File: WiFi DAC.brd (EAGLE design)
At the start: 65 x 30 mm, 27 parts

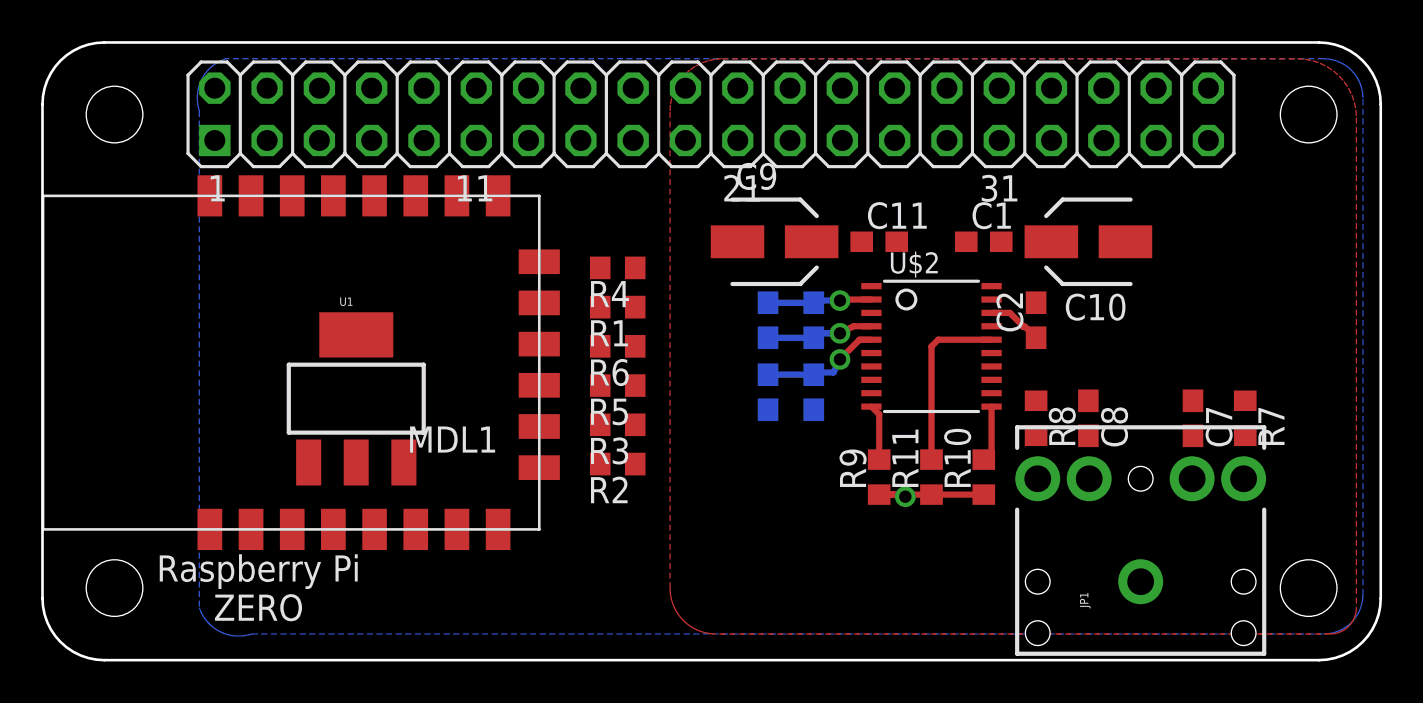
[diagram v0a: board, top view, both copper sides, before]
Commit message: test
jup
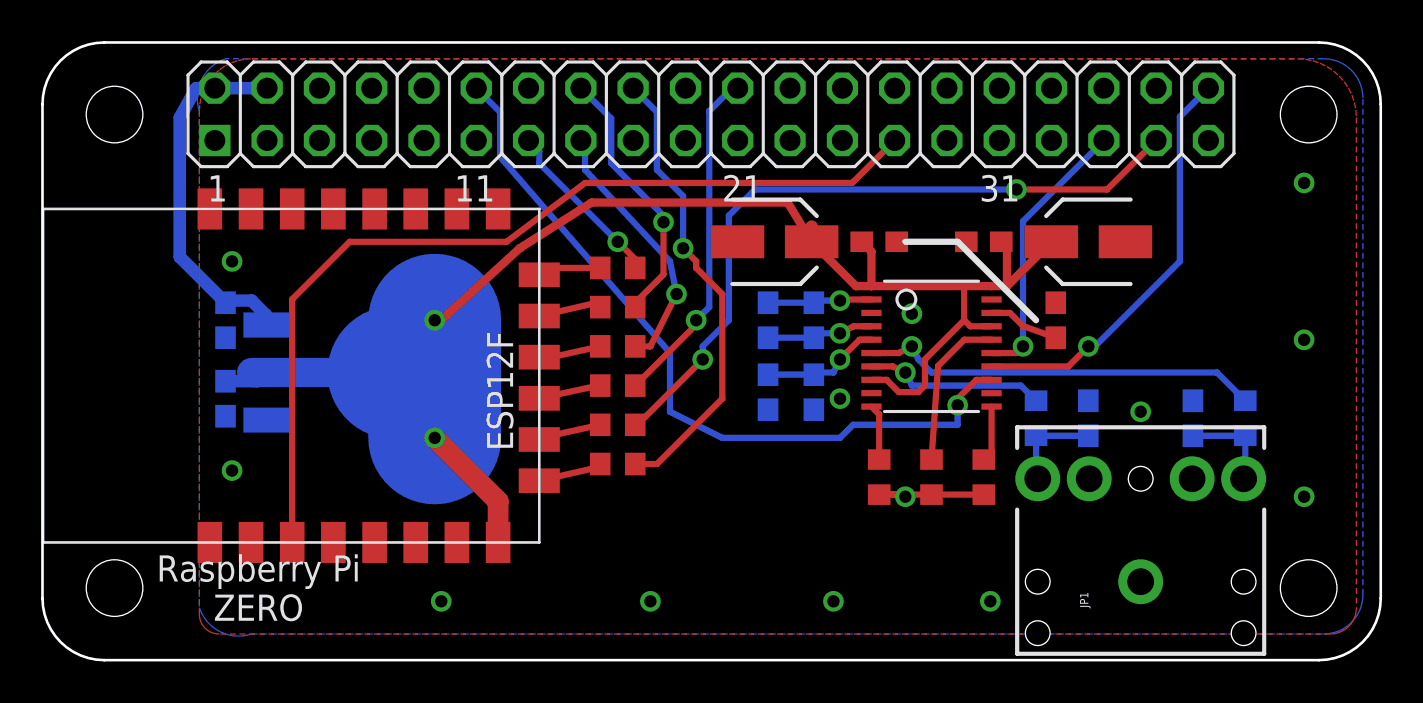
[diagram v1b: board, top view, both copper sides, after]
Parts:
- added C12: 2x 100nF, rcl:C0603
- added C13: 100nF, rcl:C0603
- C11: value 100nF -> 3x 100nF
- C4: value 100nF -> 2x 100nF
- C5: value 2.2uF -> 2x 2.2uF
- R2: value 33 -> 6x 33
- R4: value 33 -> 6x 33R
- R9: value 47k -> 3x 47k
- moved U1 1.80 mm to (14.0, 14.0), flipped to the bottom, turned to 90 degrees
- moved C2 0.95 mm to (49.2, 16.5)
- moved MDL1 0.63 mm to (24.1, 5.71)
- turned C1 to 180 degrees
- flipped C7 to the bottom
- flipped C8 to the bottom
- flipped R7 to the bottom
- flipped R8 to the bottom
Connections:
- net +3V3: now also C12.1
- net +5V: now also C13.1
- net GND: now also C12.2, C13.2
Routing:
- net +3V3: track 0.00 -> 82.6 mm, vias 0 -> 2
- net N$13: track 0.00 -> 44.0 mm
- net N$16: track 0.00 -> 37.1 mm, vias 0 -> 1
- net N$9: track 0.00 -> 34.4 mm, vias 0 -> 2
- net N$8: track 0.00 -> 22.4 mm, vias 0 -> 1
- net N$15: track 0.00 -> 20.2 mm, vias 0 -> 1
- net N$23: track 0.00 -> 19.5 mm, vias 0 -> 1
- net +5V: track 0.00 -> 17.8 mm
- net N$11: track 0.00 -> 16.7 mm, vias 0 -> 1
- net N$14: track 0.00 -> 13.3 mm, vias 0 -> 1
- net N$7: track 0.00 -> 12.9 mm, vias 0 -> 1
- net N$12: track 0.00 -> 12.8 mm, vias 0 -> 1
- net N$24: track 0.00 -> 8.76 mm, vias 0 -> 1
- net N$10: track 0.00 -> 8.34 mm, vias 0 -> 1
- net N$22: track 0.00 -> 4.66 mm
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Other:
- board text added: "ESP12F"
- board text added: "LM1117-3.3"
